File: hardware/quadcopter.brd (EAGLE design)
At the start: 126.2 x 126.2 mm, 85 parts, among them J1 AVR_SPI_PRG_6-SMD, J2 HEADER-4POS-0.1IN-FEMALE-SMD-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, J3 HEADER-10POSTH-254X10, J4 HEADER-4POS-0.1IN-FEMALE-SMD-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, M1 MOTOR_PADS_GND-MOLEX-SMD, M2 MOTOR_PADS_GND-MOLEX-SMD, M3 MOTOR_PADS_GND-MOLEX-SMD, M4 MOTOR_PADS_GND-MOLEX-SMD, Q1 MOSFET-SI2302CDS-T1-E3CT-ND, Q2 MOSFET-SI2302CDS-T1-E3CT-ND, Q3 MOSFET-SI2302CDS-T1-E3CT-ND, Q4 MOSFET-SI2302CDS-T1-E3CT-ND, Q5 MOSFET-SI2302CDS-T1-E3CT-ND, Q6 MOSFET-SI2302CDS-T1-E3CT-ND, Q7 MOSFET-SI2302CDS-T1-E3CT-ND, Q8 MOSFET-SI2302CDS-T1-E3CT-ND, Q9 MOSFET-SI2302CDS-T1-E3CT-ND, SW1 PUSHBUTTON_SMD-VERTICAL-1, U1 ATMEGA128RFA1, U2 LSM-IMU-497-18367-1-NDIMU, Y1 CRYSTAL5X3

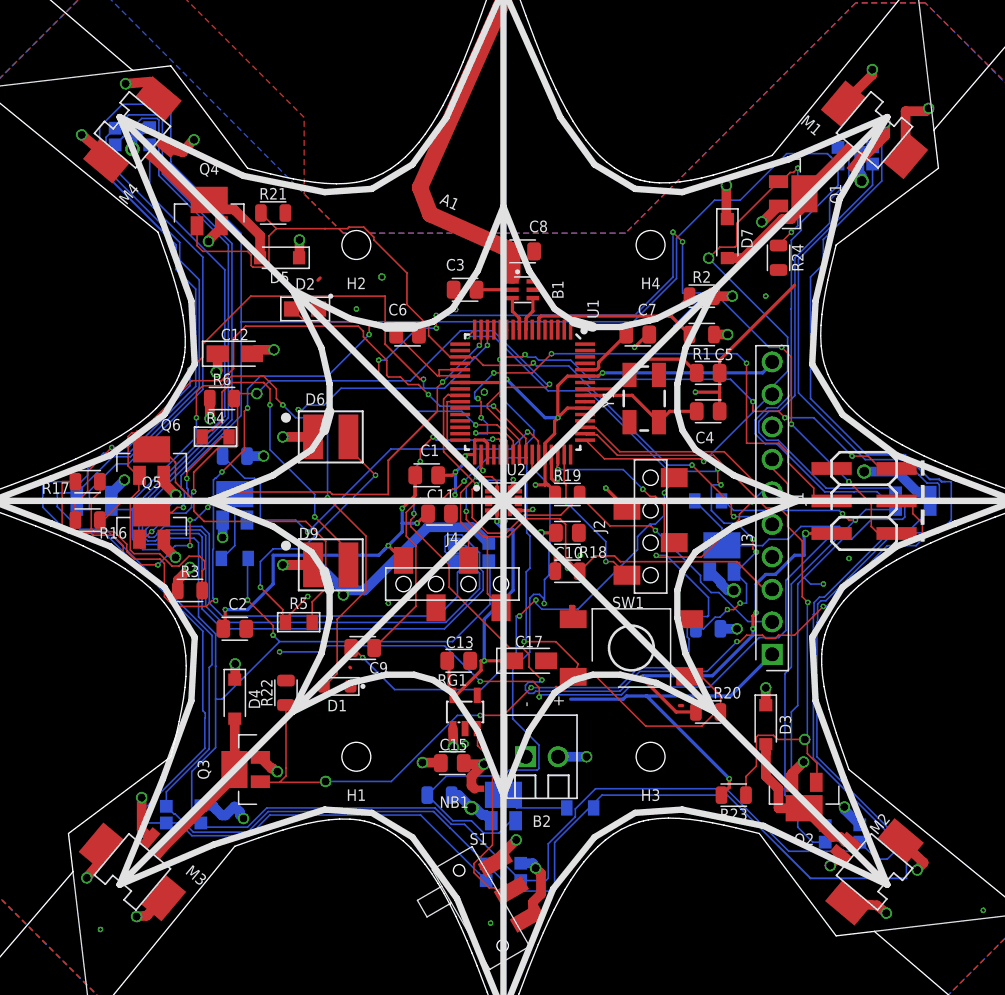
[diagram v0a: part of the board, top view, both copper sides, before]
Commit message: fixed quick check
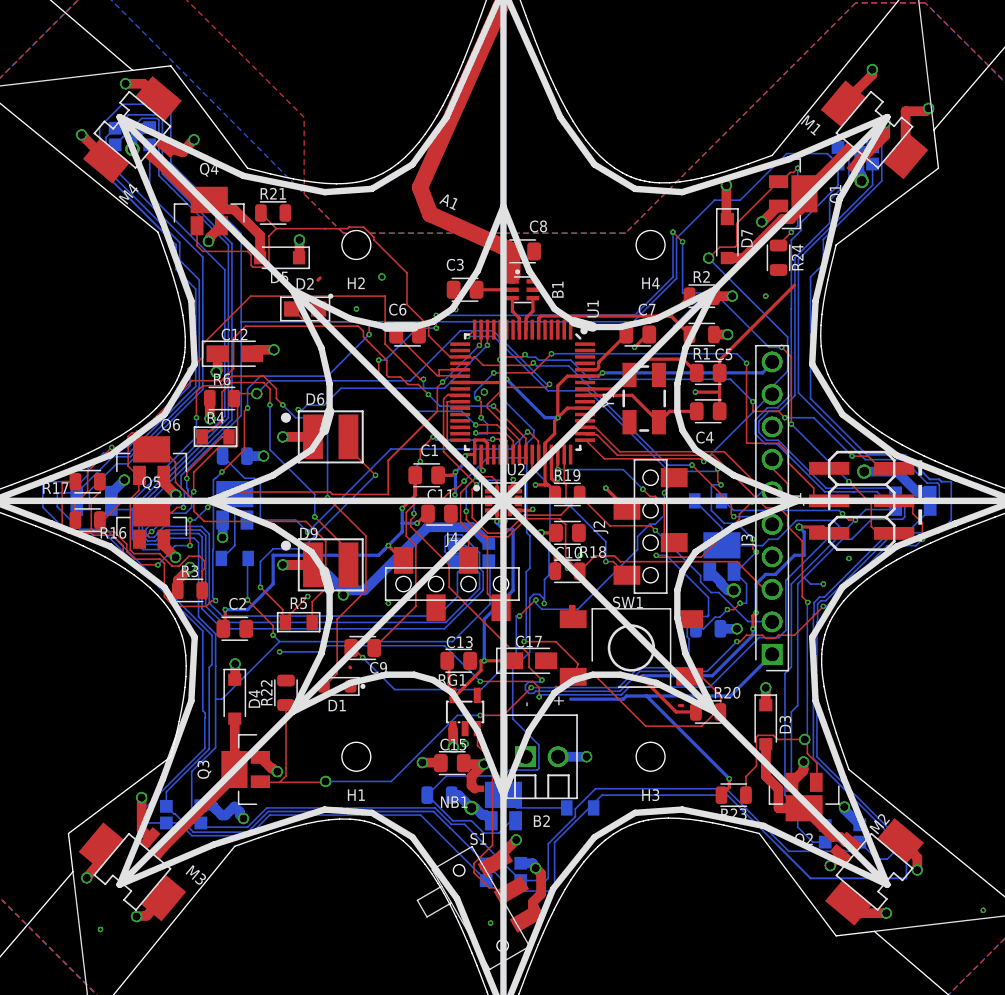
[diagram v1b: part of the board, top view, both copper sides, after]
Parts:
- moved J1 0.19 mm to (28.0, 0.00)
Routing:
- net BAT_GND: track 62.9 -> 61.2 mm
- net 3V: track 123.8 -> 125.0 mm

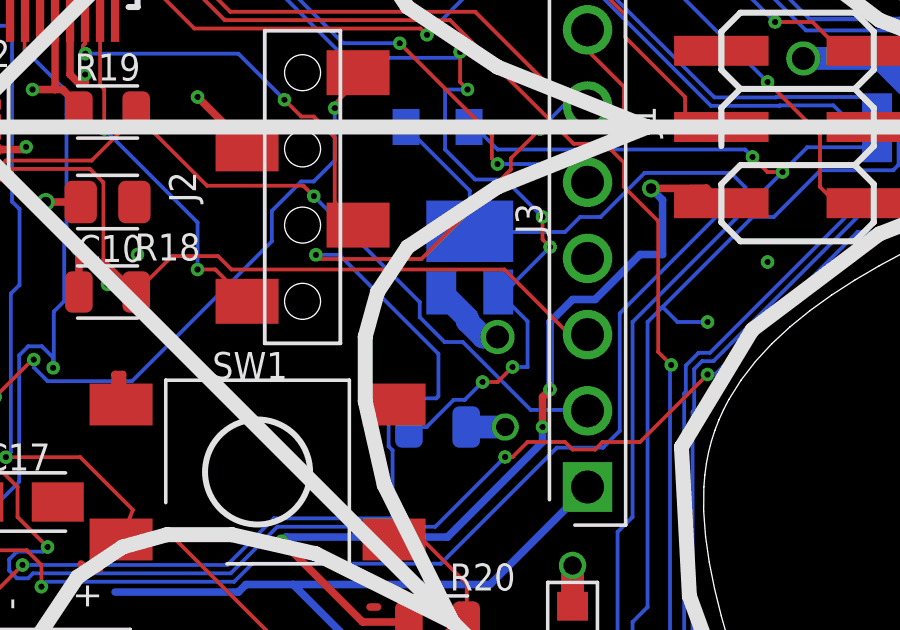
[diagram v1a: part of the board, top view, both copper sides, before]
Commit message: fixed quick check 2
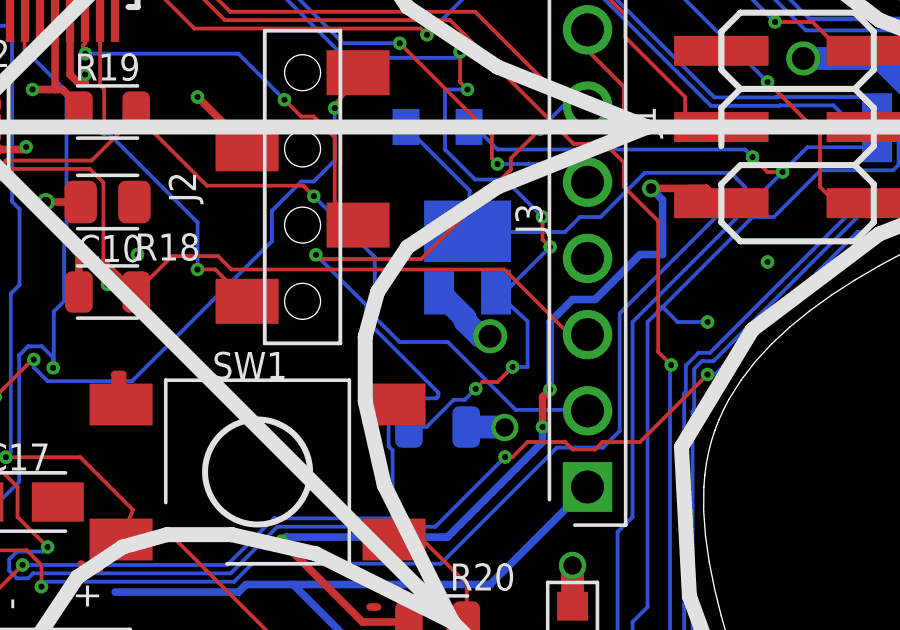
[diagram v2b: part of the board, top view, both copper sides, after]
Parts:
- moved Q7 0.07 mm to (17.0, -4.50)
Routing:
- net SCL: track 51.6 -> 52.5 mm
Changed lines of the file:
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@@
 <attribute name="VALUE" x="-29.5" y="-2.5" size="0.9" layer="28" font="vector" rot="MR0"/>
 </element>
-<element name="Q7" library="custom_" library_urn="urn:adsk.wipprod:fs.file:vf.FjMADskDQ2Se9fX1PD5xcw" package="SOT95P240X110-3MOSFET" value="MOSFET-SI2302CDS-T1-E3CT-ND" x="17.0726" y="-4.5" smashed="yes" rot="MR0">
-<attribute name="CREATOR" value="ELENA" x="23.0726" y="3.5" size="1.778" layer="28" rot="MR0" display="off"/>
-<attribute name="DIST" value="Digikey" x="23.0726" y="3.5" size="1.778" layer="28" rot="MR0" display="off"/>
-<attribute name="DISTPN" value="SI2302CDS-T1-E3CT-ND" x="23.0726" y="3.5" size="1.778" layer="28" rot="MR0" display="off"/>
-<attribute name="NAME" x="17.5726" y="-1.5" size="0.9" layer="26" font="vector" rot="MR0" align="bottom-center"/>
+<element name="Q7" library="custom_" library_urn="urn:adsk.wipprod:fs.file:vf.FjMADskDQ2Se9fX1PD5xcw" package="SOT95P240X110-3MOSFET" value="MOSFET-SI2302CDS-T1-E3CT-ND" x="17" y="-4.5" smashed="yes" rot="MR0">
+<attribute name="CREATOR" value="ELENA" x="23" y="3.5" size="1.778" layer="28" rot="MR0" display="off"/>
+<attribute name="DIST" value="Digikey" x="23" y="3.5" size="1.778" layer="28" rot="MR0" display="off"/>
+<attribute name="DISTPN" value="SI2302CDS-T1-E3CT-ND" x="23" y="3.5" size="1.778" layer="28" rot="MR0" display="off"/>
+<attribute name="NAME" x="17.5" y="-1.5" size="0.9" layer="26" font="vector" rot="MR0" align="bottom-center"/>
 </element>
 <element name="R7" library="quadparts_prebuilt_2022" package="RESC2012X60_HS" value="10K" x="16" y="-10" smashed="yes" rot="MR0">
@@
 <wire x1="21.5" y1="23.05" x2="20.26176875" y2="21.81176875" width="0.762" layer="1"/>
 <wire x1="20.26176875" y1="21.81176875" x2="20.18623125" y2="21.81176875" width="0.762" layer="1"/>
-<wire x1="16.955" y1="-10" x2="18.2546" y2="-10" width="0.762" layer="16"/>
 <wire x1="-20.045" y1="3.5" x2="-18.7454" y2="3.5" width="0.762" layer="16"/>
 <wire x1="-21.95" y1="-1.5" x2="-21.95" y2="-2.8596" width="0.762" layer="16"/>
-<via x="18.2546" y="-10" extent="1-16" drill="0.6096">
-</via>
 <via x="-18.7454" y="3.5" extent="1-16" drill="0.6096">
 </via>
@@
 <wire x1="-2.5" y1="-24" x2="-2.20434375" y2="-24" width="0.762" layer="16"/>
 <wire x1="-2.20434375" y1="-24" x2="-1.67094375" y2="-24.5334" width="0.762" layer="16"/>
-<via x="18" y="-7" extent="1-16" drill="0.762">
-</via>
-<wire x1="16.1226" y1="-5.5" x2="16.9892" y2="-6.3666" width="0.762" layer="16"/>
-<wire x1="16.9892" y1="-6.3666" x2="16.9892" y2="-6.47094375" width="0.762" layer="16"/>
-<wire x1="16.9892" y1="-6.47094375" x2="17.51825625" y2="-7" width="0.762" layer="16"/>
-<wire x1="17.51825625" y1="-7" x2="18" y2="-7" width="0.762" layer="16"/>
+<via x="17.75" y="-6.9739" extent="1-16" drill="0.762">
+</via>
 <via x="-17.67299375" y="-21.16489375" extent="1-16" drill="0.6096">
 </via>
@@
 <wire x1="-22.9166" y1="20.52905625" x2="-22.9166" y2="20.6334" width="0.762" layer="1"/>
 <wire x1="-22.9166" y1="20.6334" x2="-22.05" y2="21.5" width="0.762" layer="1"/>
+<via x="18.23839375" y="-10.01620625" extent="1-16" drill="0.6096">
+</via>
+<wire x1="16.955" y1="-10" x2="18.2221875" y2="-10" width="0.762" layer="16"/>
+<wire x1="18.2221875" y1="-10" x2="18.23839375" y2="-10.01620625" width="0.762" layer="16"/>
+<wire x1="16.05" y1="-5.5" x2="16.9166" y2="-6.3666" width="0.762" layer="16"/>
+<wire x1="16.9166" y1="-6.3666" x2="16.9166" y2="-6.47094375" width="0.762" layer="16"/>
+<wire x1="16.9166" y1="-6.47094375" x2="17.41955625" y2="-6.9739" width="0.762" layer="16"/>
+<wire x1="17.41955625" y1="-6.9739" x2="17.75" y2="-6.9739" width="0.762" layer="16"/>
 </signal>
 <signal name="PWM2">
@@
 <wire x1="10.5444125" y1="-13.0444125" x2="8.990175" y2="-14.59865" width="0.127" layer="16"/>
 <wire x1="8.990175" y1="-14.59865" x2="2.16535" y2="-14.59865" width="0.127" layer="16"/>
-<wire x1="16.028825" y1="-7.56" x2="12.729675" y2="-4.26085" width="0.127" layer="16"/>
-<wire x1="11.94435" y1="-4.26085" x2="12.729675" y2="-4.26085" width="0.127" layer="16"/>
-<wire x1="16.028825" y1="-7.56" x2="16.028825" y2="-8.971175" width="0.127" layer="16"/>
 <wire x1="16.028825" y1="-8.971175" x2="16" y2="-9" width="0.127" layer="16"/>
 <wire x1="16" y1="-9" x2="15.9555875" y2="-9.0444125" width="0.127" layer="16"/>
@@
 <wire x1="14.5" y1="-13" x2="14.4555875" y2="-13.0444125" width="0.127" layer="16"/>
 <wire x1="14.4555875" y1="-13.0444125" x2="10.5444125" y2="-13.0444125" width="0.127" layer="16"/>
+<wire x1="11.94435" y1="-4.26085" x2="13.6273" y2="-5.9438" width="0.127" layer="16"/>
+<wire x1="13.6273" y1="-5.9438" x2="13.6273" y2="-6.45516875" width="0.127" layer="16"/>
+<wire x1="16.028825" y1="-8.85669375" x2="16.028825" y2="-8.971175" width="0.127" layer="16"/>
+<wire x1="13.6273" y1="-6.45516875" x2="16.028825" y2="-8.85669375" width="0.127" layer="16"/>
 </signal>
 <signal name="PWM4">
@@
 <wire x1="-2.0955" y1="1.2573" x2="-2.4445" y2="0.9083" width="0.127" layer="1"/>
 <wire x1="-2.4445" y1="0.9083" x2="-2.4445" y2="-1.31291875" width="0.127" layer="1"/>
-<wire x1="11.8745" y1="-2.30505" x2="15.4067" y2="-5.83725" width="0.127" layer="16"/>
-<wire x1="15.4067" y1="-5.83725" x2="15.4067" y2="-6.33943125" width="0.127" layer="16"/>
-<wire x1="19.10385625" y1="-9.42975" x2="20.955" y2="-9.42975" width="0.127" layer="16"/>
+<wire x1="11.8745" y1="-2.30505" x2="13.9067" y2="-4.33725" width="0.127" layer="16"/>
+<wire x1="13.9067" y1="-4.33725" x2="13.9067" y2="-6.33943125" width="0.127" layer="16"/>
+<wire x1="18.60385625" y1="-9.42975" x2="20.955" y2="-9.42975" width="0.127" layer="16"/>
 <wire x1="-3.3491" y1="-1.65391875" x2="-2.73" y2="-2.27301875" width="0.127" layer="1"/>
 <wire x1="-2.73" y1="-2.27301875" x2="-2.73" y2="-4.65" width="0.127" layer="1"/>
@@
 <wire x1="-4.67995" y1="7.9629" x2="-4.67995" y2="3.84175" width="0.127" layer="1"/>
 <wire x1="-4.67995" y1="3.84175" x2="-2.409825" y2="1.571625" width="0.127" layer="1"/>
-<wire x1="15.4067" y1="-6.33943125" x2="16.23436875" y2="-7.1671" width="0.127" layer="16"/>
-<wire x1="16.23436875" y1="-7.1671" x2="16.84120625" y2="-7.1671" width="0.127" layer="16"/>
-<wire x1="16.84120625" y1="-7.1671" x2="19.10385625" y2="-9.42975" width="0.127" layer="16"/>
+<wire x1="13.9067" y1="-6.33943125" x2="14.73436875" y2="-7.1671" width="0.127" layer="16"/>
+<wire x1="14.73436875" y1="-7.1671" x2="16.34120625" y2="-7.1671" width="0.127" layer="16"/>
+<wire x1="16.34120625" y1="-7.1671" x2="18.60385625" y2="-9.42975" width="0.127" layer="16"/>
 </signal>
 <signal name="SDA">
@@
 <wire x1="-17.493" y1="-11.80465" x2="-14.2565625" y2="-11.80465" width="0.127" layer="16"/>
 <wire x1="14.95" y1="0" x2="17.0726" y2="-2.1226" width="0.127" layer="16"/>
-<wire x1="17.0726" y1="-2.1226" x2="17.0726" y2="-3.475" width="0.127" layer="16"/>
+<wire x1="17.0726" y1="-2.1226" x2="17" y2="-3.475" width="0.127" layer="16"/>
 <wire x1="17.25" y1="-3.5" x2="20.25" y2="-3.5" width="0.127" layer="16"/>
 <wire x1="20.25" y1="-3.5" x2="20.75" y2="-3" width="0.127" layer="16"/>
-<wire x1="17.0726" y1="-3.475" x2="17.25" y2="-3.5" width="0.127" layer="16"/>
+<wire x1="17" y1="-3.475" x2="17.25" y2="-3.5" width="0.127" layer="16"/>
 <via x="2.794" y="-15.32255" extent="1-16" drill="0.2032">
 </via>
@@
 <via x="18.5" y="-8" extent="1-16" drill="0.2032">
 </via>
-<via x="17.5" y="-8.5" extent="1-16" drill="0.2032">
-</via>
-<wire x1="19" y1="-6.4774" x2="18.0226" y2="-5.5" width="0.127" layer="16"/>
+<wire x1="19" y1="-6.4774" x2="17.95" y2="-5.5" width="0.127" layer="16"/>
 <wire x1="19" y1="-8" x2="19" y2="-6.4774" width="0.127" layer="16"/>
 <wire x1="19" y1="-8" x2="18.5" y2="-8" width="0.127" layer="16"/>
-<wire x1="17.5" y1="-8.5" x2="16.9059" y2="-9.0941" width="0.127" layer="16"/>
-<wire x1="16.9059" y1="-9.0941" x2="16.5403" y2="-9.0941" width="0.127" layer="16"/>
-<wire x1="15.6344" y1="-10" x2="15.045" y2="-10" width="0.127" layer="16"/>
-<wire x1="16.5403" y1="-9.0941" x2="15.6344" y2="-10" width="0.127" layer="16"/>
+<wire x1="16.5403" y1="-9.0941" x2="16.9059" y2="-9.0941" width="0.127" layer="16"/>
+<wire x1="15.045" y1="-10" x2="15.6344" y2="-10" width="0.127" layer="16"/>
+<wire x1="15.6344" y1="-10" x2="16.5403" y2="-9.0941" width="0.127" layer="16"/>
 <wire x1="18.5" y1="-8" x2="18" y2="-8.5" width="0.127" layer="1"/>
 <wire x1="18" y1="-8.5" x2="17.5" y2="-8.5" width="0.127" layer="1"/>
@@
 <wire x1="16.75" y1="2.5" x2="16.75" y2="1.5" width="0.127" layer="1"/>
 <wire x1="16.75" y1="2.30505" x2="16.75" y2="2.5" width="0.127" layer="16"/>
-<wire x1="18.25" y1="-5.5" x2="18.0226" y2="-5.5" width="0.127" layer="16"/>
+<wire x1="18.25" y1="-5.5" x2="17.95" y2="-5.5" width="0.127" layer="16"/>
 <via x="19.75" y="-4" extent="1-16" drill="0.2032">
 </via>
@@
 <via x="16.75" y="2.5" extent="1-16" drill="0.2032">
 </via>
+<via x="17.2727375" y="-8.7272625" extent="1-16" drill="0.2032">
+</via>
+<wire x1="17.5" y1="-8.5" x2="17.2727375" y2="-8.7272625" width="0.127" layer="1"/>
+<wire x1="16.9059" y1="-9.0941" x2="17.2727375" y2="-8.7272625" width="0.127" layer="16"/>
 </signal>
 <signal name="PB6">
